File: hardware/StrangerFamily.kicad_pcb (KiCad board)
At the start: 2 copper layers, 90 x 50 mm, 22 parts, among them J1 LCD_Conn, J2 Power_LEDs, J3 Output_LED, J5 Raspberry_Pi_zero, Q2 BSS138, Q3 BSS138, Q4 BSS138, U1 74LVC2T45DC, U2 74LVC1G3157

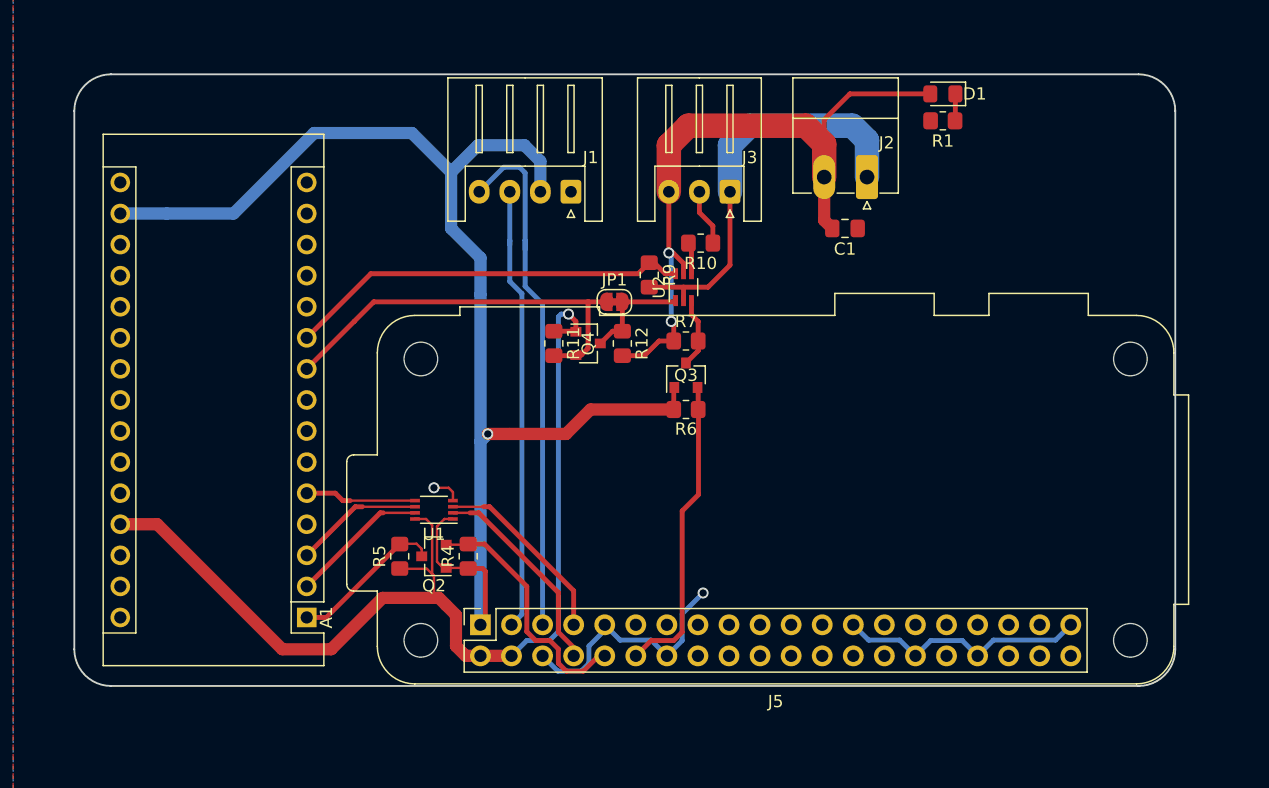
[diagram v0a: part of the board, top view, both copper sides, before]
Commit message: v2 : use logos, move footprints
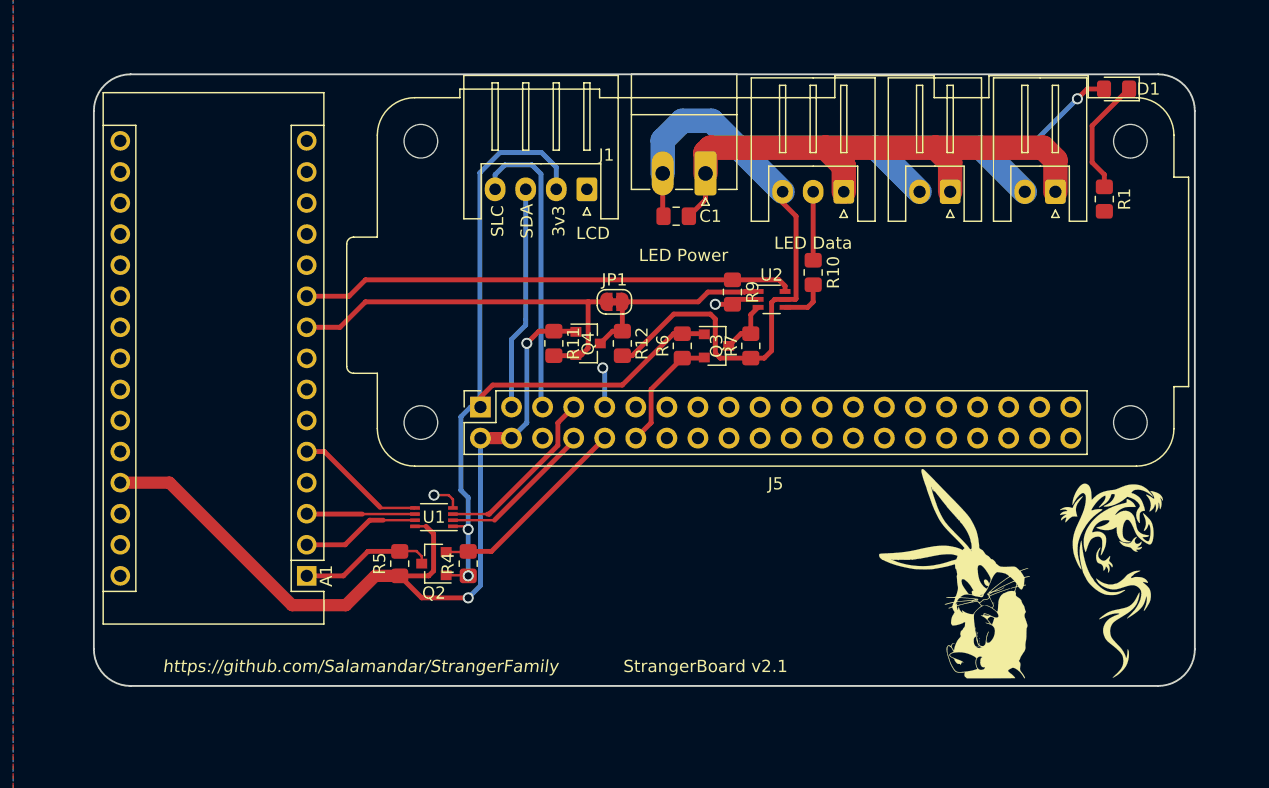
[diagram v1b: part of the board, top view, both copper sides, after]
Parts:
- added G***: LOGO, stranger_family_lib:logo_klorydryk, F.Cu at (237.2, 110.6)
- added G***: LOGO, stranger_family_lib:logo_salamandar, F.Cu at (249.4, 111.2)
- added J4: LED_Out2, Connector_JST:JST_XH_S2B-XH-A_1x02_P2.50mm_Horizontal, F.Cu at (236.6, 79.6)
- added J6: LED_Out2, Connector_JST:JST_XH_S2B-XH-A_1x02_P2.50mm_Horizontal, F.Cu at (245.2, 79.6)
- moved J5 17.8 mm to (198.2, 97.2)
- moved R1 14.7 mm to (249.2, 80.2), turned to 270 degrees
- moved D1 14.2 mm to (250.2, 71.2)
- moved C1 13.8 mm to (214.2, 81.6)
- moved J2 13.2 mm to (216.6, 78.1)
- moved R10 9.51 mm to (225.4, 86.2), turned to 270 degrees
- moved J3 9.30 mm to (227.9, 79.6)
- moved U2 7.27 mm to (222.0, 88.4), turned to 0 degrees
- moved R9 6.94 mm to (218.8, 87.8)
- moved R7 5.32 mm to (220.3, 92.2), turned to 90 degrees
- moved R6 5.21 mm to (214.7, 92.2), turned to 270 degrees
- moved Q3 3.47 mm to (217.5, 92.2), turned to 0 degrees
- moved A1 3.40 mm to (184.0, 111.0)
- moved J1 1.32 mm to (206.9, 79.4)
- moved U1 0.60 mm to (194.4, 106.2)
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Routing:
- net +3V3: track 112.3 -> 68.0 mm, vias 1 -> 2
- net VCC: track 56.0 -> 93.4 mm, vias 2 -> 1
- net GND: track 77.7 -> 55.2 mm, vias 2 -> 3
- net /LCD_SLC: track 43.1 -> 24.7 mm
- net /LCD_SDA: track 36.5 -> 18.3 mm
- net +5V: track 87.1 -> 70.8 mm, vias 1 -> 2
- net /PWM0: track 25.2 -> 9.93 mm
- net Net-(D1-Pad1): track 2.20 -> 9.68 mm
- net /Arduino_is_out: track 33.1 -> 40.3 mm
- net /Arduino_out_VDD: track 9.01 -> 16.1 mm
- net /RPi_RX: track 21.4 -> 16.8 mm
- net /RPi_TX: track 17.0 -> 12.8 mm
- net /RX_enable: track 9.10 -> 10.9 mm
- net /Nano_RX: track 11.3 -> 9.68 mm
- net /Nano_TX: track 12.7 -> 11.0 mm
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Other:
- board text added: "3v3"
- board text added: "LCD"
- board text added: "LED Data"
- board text added: "LED Power"
- board text added: "SDA"
- board text added: "SLC"
- board text added: "StrangerBoard v2.1"
- board text added: "https://github.com/Salamandar/StrangerFamily"
